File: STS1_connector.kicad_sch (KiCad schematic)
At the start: 4 parts, among them J1 Conn_02x20_Odd_Even, J2 Conn_02x20_Odd_Even

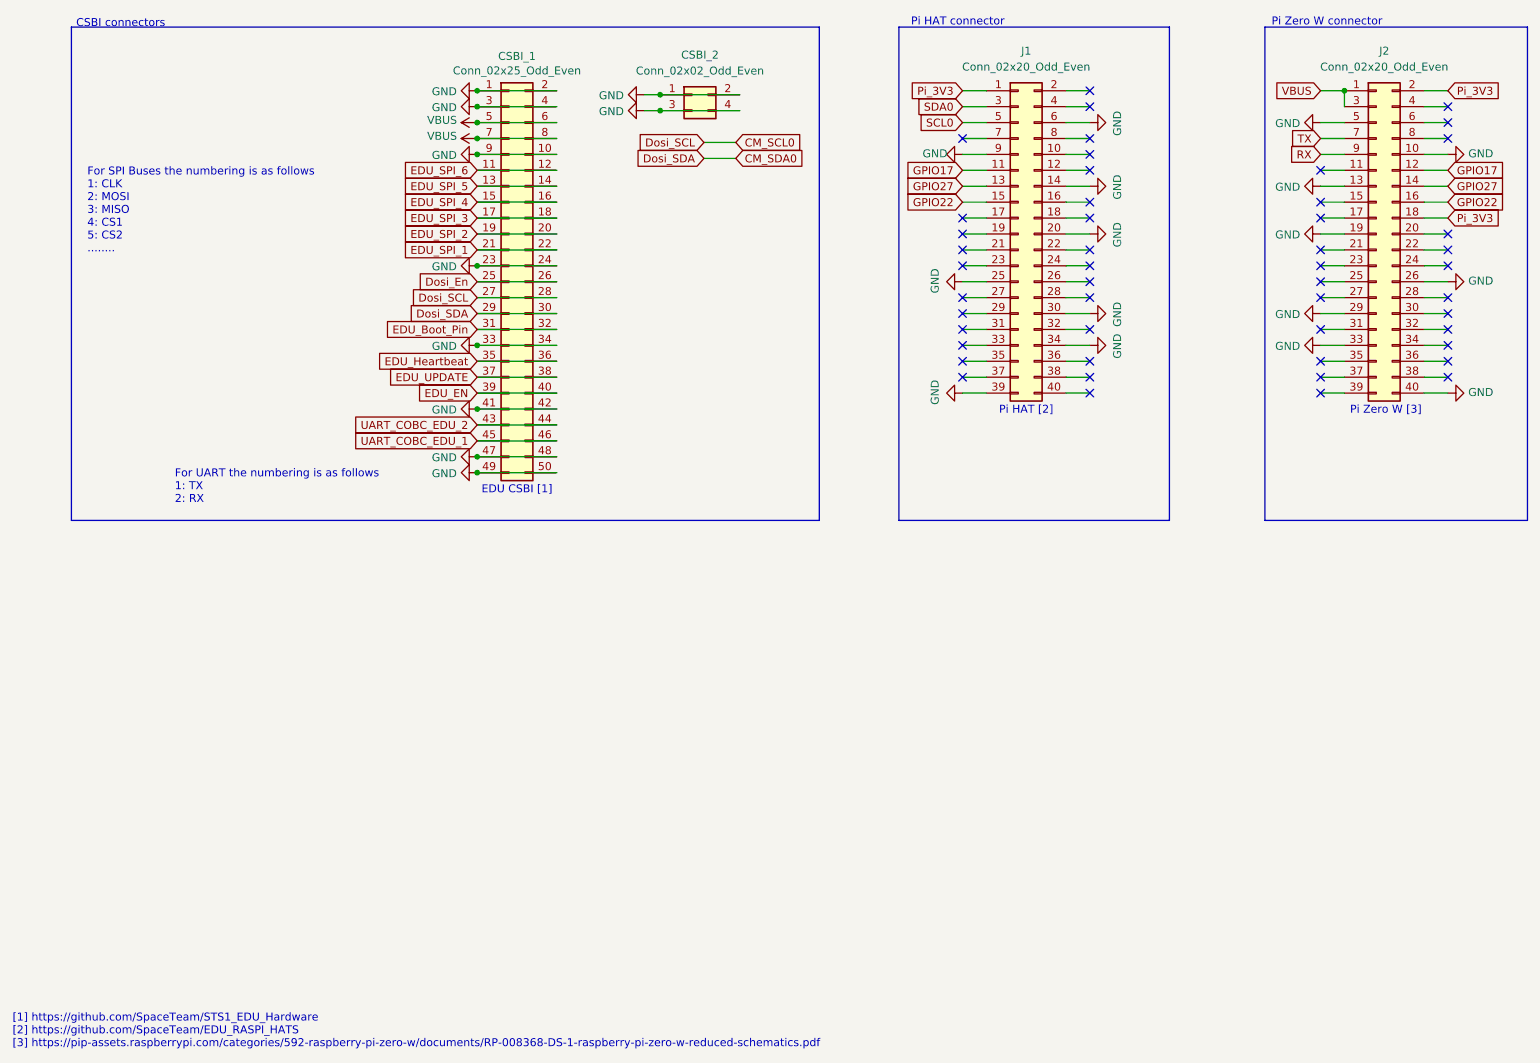
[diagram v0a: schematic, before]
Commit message: Finilize connection and placement of components
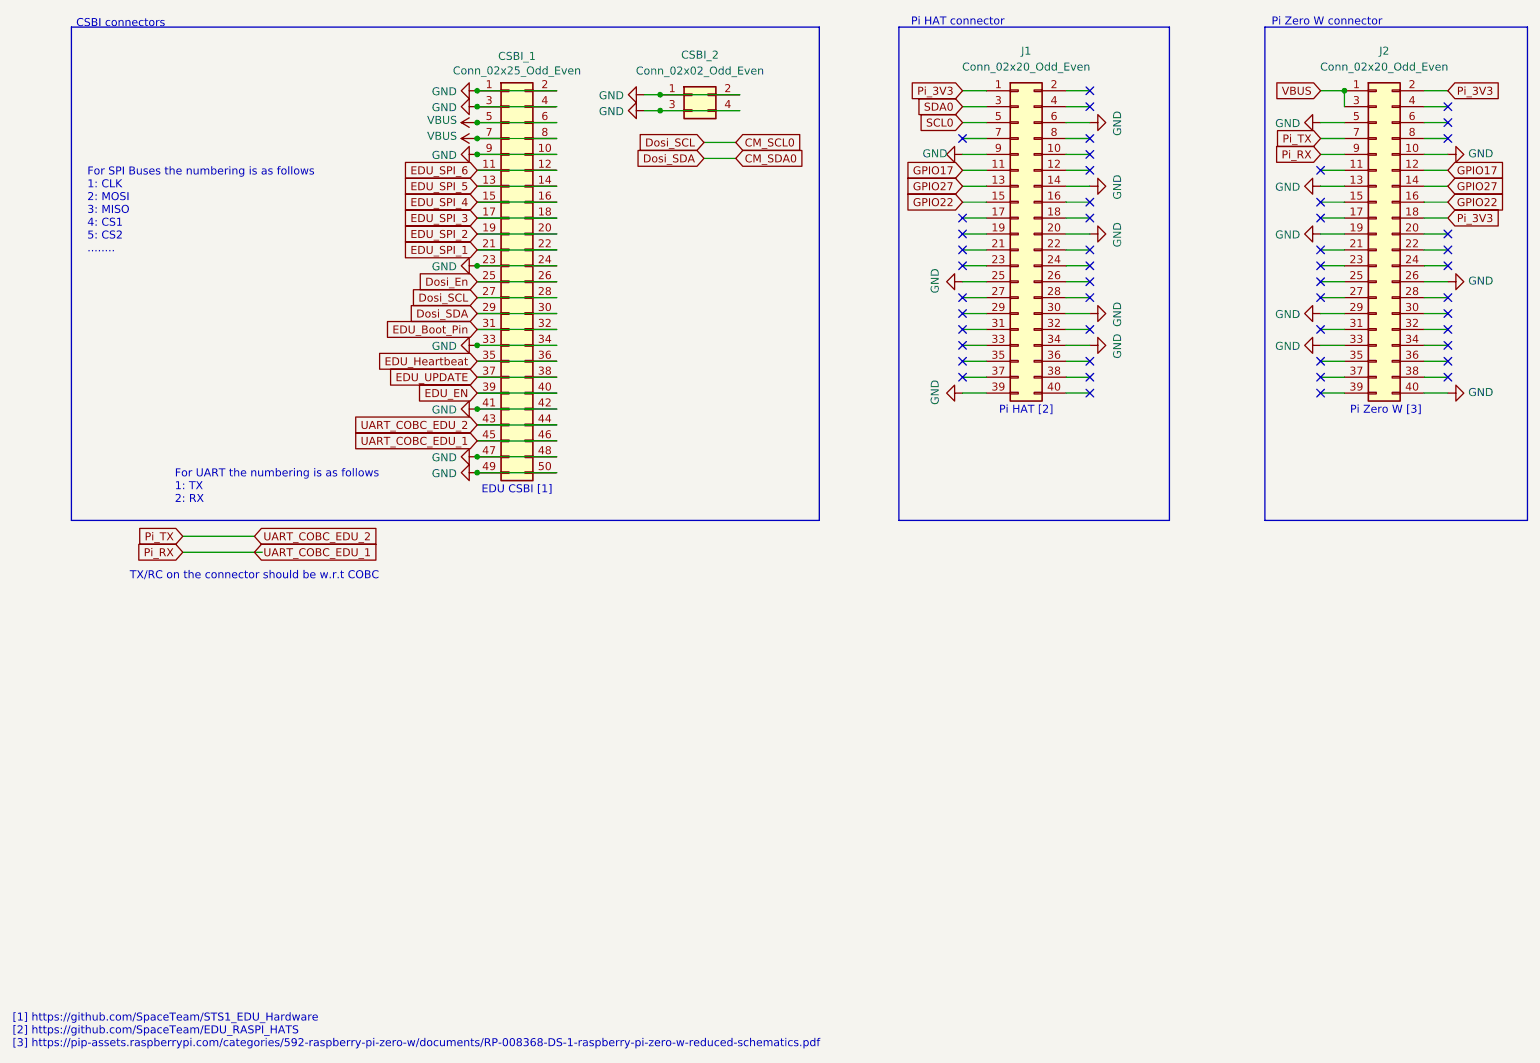
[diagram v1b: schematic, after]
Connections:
- net UART_COBC_EDU_1 is gone; now on net Pi_RX: CSBI_1.45 (Pin_45), CSBI_1.46 (Pin_46)
- net UART_COBC_EDU_2 is gone; now on net Pi_TX: CSBI_1.43 (Pin_43), CSBI_1.44 (Pin_44)
- net RX renamed Pi_RX
- net TX renamed Pi_TX
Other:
- note added: "TX/RC on the connector should be w.r.t COBC"
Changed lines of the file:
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@@
 		)
 	)
+	(text "TX/RC on the connector should be w.r.t COBC"
+		(exclude_from_sim no)
+		(at 52.07 121.92 0)
+		(effects
+			(font
+				(size 1.27 1.27)
+			)
+		)
+	)
 	(text "Pi HAT connector"
 		(exclude_from_sim no)
@@
 	(wire
 		(pts
+			(xy 40.64 118.11) (xy 53.34 118.11)
+		)
+		(stroke
+			(width 0)
+			(type default)
+		)
+	)
+	(wire
+		(pts
 			(xy 238.76 85.09) (xy 242.57 85.09)
 		)
@@
 	(wire
 		(pts
+			(xy 40.64 115.57) (xy 52.07 115.57)
+		)
+		(stroke
+			(width 0)
+			(type default)
+		)
+	)
+	(wire
+		(pts
 			(xy 238.76 54.61) (xy 242.57 54.61)
 		)
@@
 		)
 	)
-	(global_label "RX"
+	(global_label "Pi_RX"
 		(shape input)
 		(at 222.25 54.61 180)
@@
 		)
 		(property "Intersheetrefs" "${INTERSHEET_REFS}"
-			(at 217.4395 54.61 0)
+			(at 214.5971 54.61 0)
 			(hide yes)
 			(show_name no)
@@
 		)
 	)
-	(global_label "TX"
+	(global_label "Pi_TX"
 		(shape input)
 		(at 222.25 52.07 180)
@@
 		)
 		(property "Intersheetrefs" "${INTERSHEET_REFS}"
-			(at 217.7419 52.07 0)
+			(at 214.8995 52.07 0)
 			(hide yes)
 			(show_name no)
@@
 		)
 	)
+	(global_label "UART_COBC_EDU_2"
+		(shape input)
+		(at 52.07 115.57 0)
+		(fields_autoplaced yes)
+		(effects
+			(font
+				(size 1.27 1.27)
+			)
+			(justify left)
+		)
+		(property "Intersheetrefs" "${INTERSHEET_REFS}"
+			(at 72.06 115.57 0)
+			(hide yes)
+			(show_name no)
+			(do_not_autoplace no)
+			(effects
+				(font
+					(size 1.27 1.27)
+				)
+				(justify left)
+			)
+		)
+	)
 	(global_label "EDU_SPI_5"
 		(shape input)
@@
 		)
 	)
+	(global_label "Pi_TX"
+		(shape input)
+		(at 40.64 115.57 180)
+		(fields_autoplaced yes)
+		(effects
+			(font
+				(size 1.27 1.27)
+			)
+			(justify right)
+		)
+		(property "Intersheetrefs" "${INTERSHEET_REFS}"
+			(at 33.2895 115.57 0)
+			(hide yes)
+			(show_name no)
+			(do_not_autoplace no)
+			(effects
+				(font
+					(size 1.27 1.27)
+				)
+				(justify right)
+			)
+		)
+	)
 	(global_label "GPIO22"
 		(shape input)
@@
 		)
 	)
+	(global_label "Pi_RX"
+		(shape input)
+		(at 40.64 118.11 180)
+		(fields_autoplaced yes)
+		(effects
+			(font
+				(size 1.27 1.27)
+			)
+			(justify right)
+		)
+		(property "Intersheetrefs" "${INTERSHEET_REFS}"
+			(at 32.9871 118.11 0)
+			(hide yes)
+			(show_name no)
+			(do_not_autoplace no)
+			(effects
+				(font
+					(size 1.27 1.27)
+				)
+				(justify right)
+			)
+		)
+	)
 	(global_label "UART_COBC_EDU_1"
 		(shape input)
@@
 		)
 	)
+	(global_label "UART_COBC_EDU_1"
+		(shape input)
+		(at 52.07 118.11 0)
+		(fields_autoplaced yes)
+		(effects
+			(font
+				(size 1.27 1.27)
+			)
+			(justify left)
+		)
+		(property "Intersheetrefs" "${INTERSHEET_REFS}"
+			(at 72.06 118.11 0)
+			(hide yes)
+			(show_name no)
+			(do_not_autoplace no)
+			(effects
+				(font
+					(size 1.27 1.27)
+				)
+				(justify left)
+			)
+		)
+	)
 	(symbol
 		(lib_id "Connector_Generic:Conn_02x25_Odd_Even")
@@
 		(in_pos_files yes)
 		(dnp no)
-		(property "Reference" "#PWR018"
+		(property "Reference" "#PWR023"
 			(at 191.77 80.01 0)
 			(hide yes)
@@
 			(project "STS1_EEE"
 				(path "/81e05c2b-9a2c-430f-84ee-6a59968cd49a/00000000-0000-0000-0000-000059c45183"
-					(reference "#PWR018")
+					(reference "#PWR023")
 					(unit 1)
 				)
@@
 		(in_pos_files yes)
 		(dnp no)
-		(property "Reference" "#PWR019"
+		(property "Reference" "#PWR022"
 			(at 191.77 67.31 0)
 			(hide yes)
@@
 			(project "STS1_EEE"
 				(path "/81e05c2b-9a2c-430f-84ee-6a59968cd49a/00000000-0000-0000-0000-000059c45183"
-					(reference "#PWR019")
+					(reference "#PWR022")
 					(unit 1)
 				)
@@
 		(in_pos_files yes)
 		(dnp no)
-		(property "Reference" "#PWR020"
+		(property "Reference" "#PWR021"
 			(at 191.77 59.69 0)
 			(hide yes)
@@
 			(project "STS1_EEE"
 				(path "/81e05c2b-9a2c-430f-84ee-6a59968cd49a/00000000-0000-0000-0000-000059c45183"
-					(reference "#PWR020")
+					(reference "#PWR021")
 					(unit 1)
 				)
@@
 		(in_pos_files yes)
 		(dnp no)
-		(property "Reference" "#PWR023"
+		(property "Reference" "#PWR018"
 			(at 158.75 74.93 0)
 			(hide yes)
@@
 			(project "STS1_EEE"
 				(path "/81e05c2b-9a2c-430f-84ee-6a59968cd49a/00000000-0000-0000-0000-000059c45183"
-					(reference "#PWR023")
+					(reference "#PWR018")
 					(unit 1)
 				)
@@
 		(in_pos_files yes)
 		(dnp no)
-		(property "Reference" "#PWR017"
+		(property "Reference" "#PWR024"
 			(at 191.77 85.09 0)
 			(hide yes)
@@
 			(project "STS1_EEE"
 				(path "/81e05c2b-9a2c-430f-84ee-6a59968cd49a/00000000-0000-0000-0000-000059c45183"
-					(reference "#PWR017")
+					(reference "#PWR024")
 					(unit 1)
 				)
@@
 		(in_pos_files yes)
 		(dnp no)
-		(property "Reference" "#PWR022"
+		(property "Reference" "#PWR017"
 			(at 158.75 54.61 0)
 			(hide yes)
@@
 			(project "STS1_EEE"
 				(path "/81e05c2b-9a2c-430f-84ee-6a59968cd49a/00000000-0000-0000-0000-000059c45183"
-					(reference "#PWR022")
+					(reference "#PWR017")
 					(unit 1)
 				)
@@
 		(in_pos_files yes)
 		(dnp no)
-		(property "Reference" "#PWR024"
+		(property "Reference" "#PWR019"
 			(at 158.75 92.71 0)
 			(hide yes)
@@
 			(project "STS1_EEE"
 				(path "/81e05c2b-9a2c-430f-84ee-6a59968cd49a/00000000-0000-0000-0000-000059c45183"
-					(reference "#PWR024")
+					(reference "#PWR019")
 					(unit 1)
 				)
@@
 		(in_pos_files yes)
 		(dnp no)
-		(property "Reference" "#PWR021"
+		(property "Reference" "#PWR020"
 			(at 191.77 49.53 0)
 			(hide yes)
@@
 			(project "STS1_EEE"
 				(path "/81e05c2b-9a2c-430f-84ee-6a59968cd49a/00000000-0000-0000-0000-000059c45183"
-					(reference "#PWR021")
+					(reference "#PWR020")
 					(unit 1)
 				)
